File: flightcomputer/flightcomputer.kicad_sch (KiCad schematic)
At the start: 82 parts, among them J1 Conn_Coaxial, J10 Conn_01x03, J11 Conn_01x03, J12 ESQ-113-14-G-D, J13 Conn_01x07, J14 S3B-PH-K-S-GW, J15 B2P-VHLFSN, J2 Conn_Coaxial, J3 Conn_Coaxial, J4 Conn_Coaxial, J5 S3B-PH-K-S-GW, J6 Conn_01x03, J7 S4B-PH-K-S_LF__SN_, J8 Conn_01x03, J9 Conn_01x06, U1 MAX-M10S, U2 LIS2MDLTR, U3 BMI088, U4 MS5607-02BA, U5 ESP32-S3-WROOM-1-N4, U6 NCP718ASNADJT1G, U7 Teensy4.1, U8 LSM6DSO32TR, U9 RFM96W-433S2

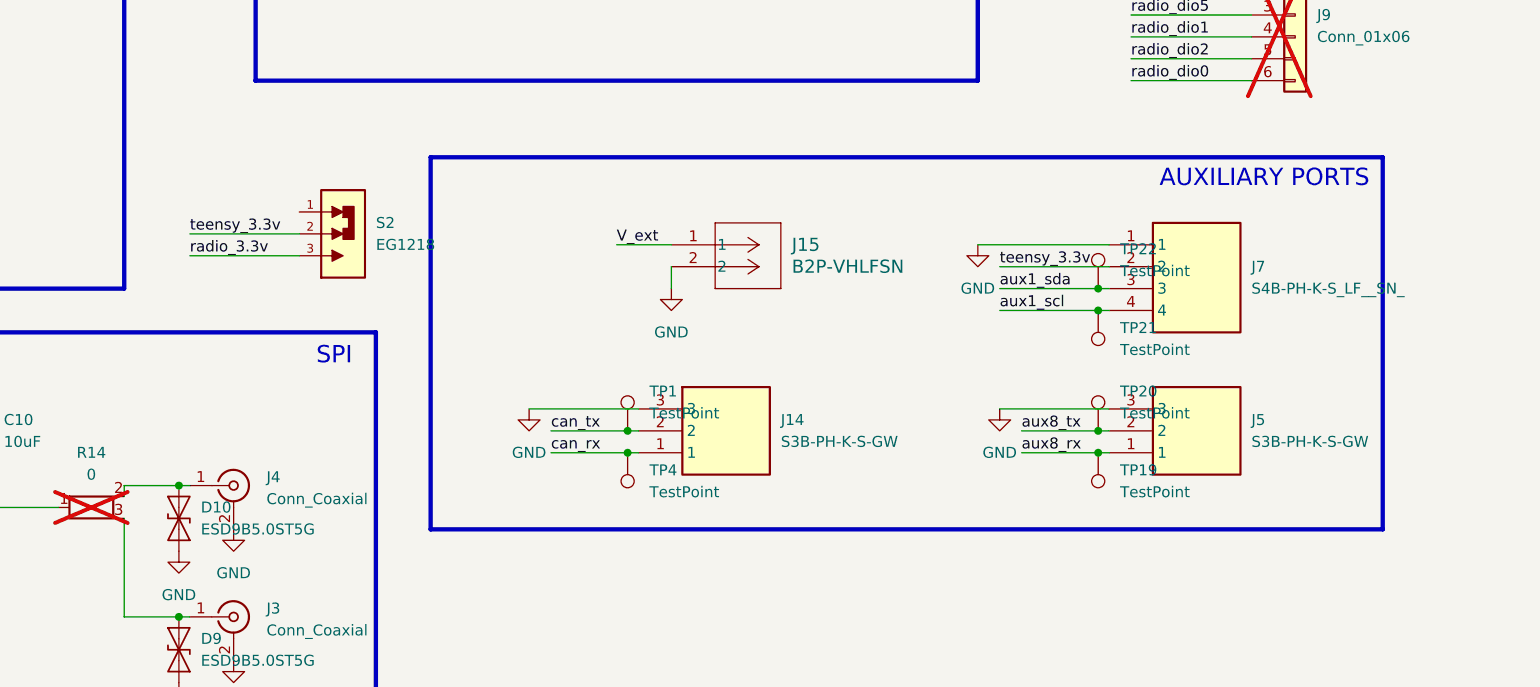
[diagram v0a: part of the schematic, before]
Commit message: prod files
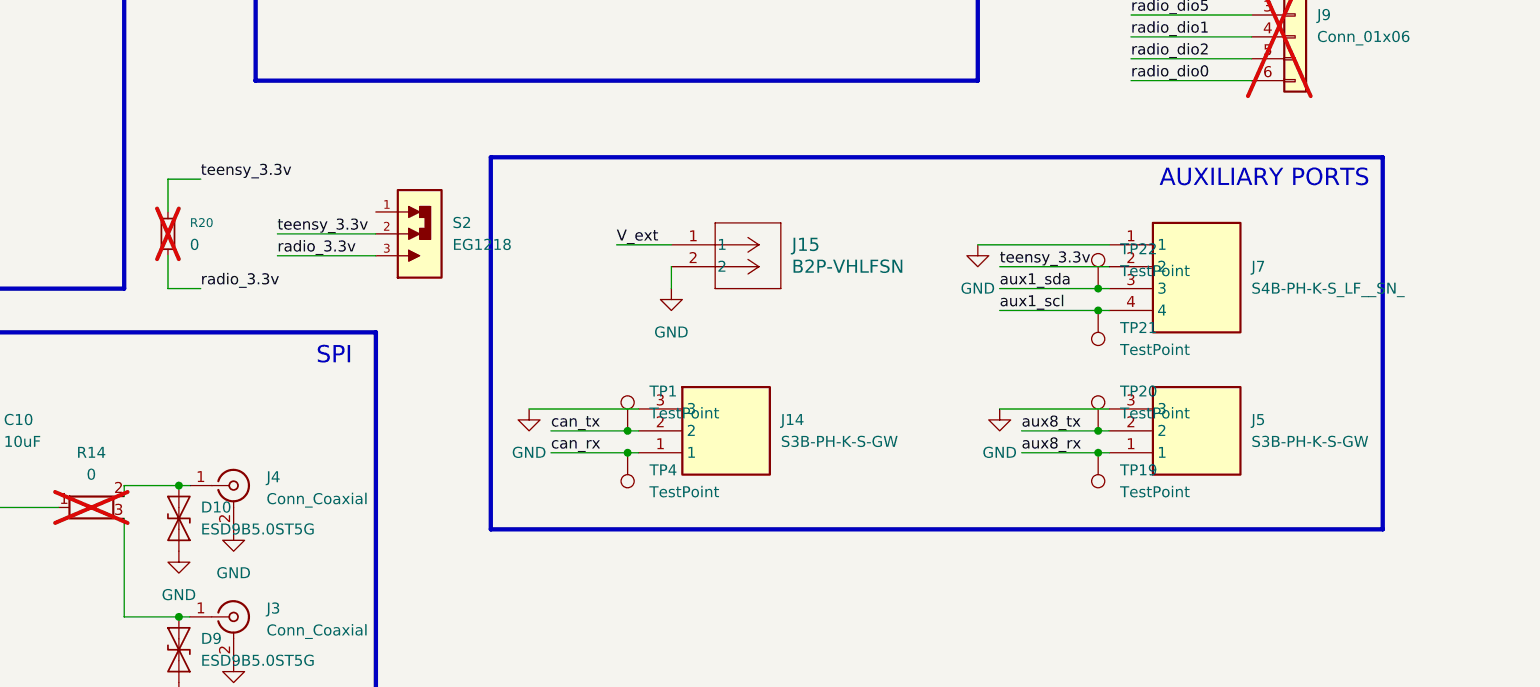
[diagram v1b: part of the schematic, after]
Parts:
- added R20: 0, Resistor_SMD:R_0603_1608Metric_Pad0.98x0.95mm_HandSolder, symbol Device:R_Small
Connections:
- net radio_3.3v: now also R20.2
- net teensy_3.3v: now also R20.1
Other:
- moved on the sheet: S2
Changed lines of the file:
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@@
 	)
 	(rectangle
-		(start 294.64 205.74)
+		(start 301.625 205.74)
 		(end 405.13 248.92)
 		(stroke
@@
 	(wire
 		(pts
-			(xy 266.7 217.17) (xy 279.4 217.17)
+			(xy 276.86 217.17) (xy 288.29 217.17)
 		)
 		(stroke
@@
 	(wire
 		(pts
+			(xy 264.16 220.98) (xy 267.97 220.98)
+		)
+		(stroke
+			(width 0)
+			(type default)
+		)
+	)
+	(wire
+		(pts
 			(xy 157.48 139.7) (xy 170.18 139.7)
 		)
@@
 	(wire
 		(pts
+			(xy 264.16 217.17) (xy 264.16 220.98)
+		)
+		(stroke
+			(width 0)
+			(type default)
+		)
+	)
+	(wire
+		(pts
 			(xy 226.06 152.4) (xy 240.03 152.4)
 		)
@@
 	(wire
 		(pts
+			(xy 264.16 208.28) (xy 267.97 208.28)
+		)
+		(stroke
+			(width 0)
+			(type default)
+		)
+	)
+	(wire
+		(pts
 			(xy 105.41 213.36) (xy 118.11 213.36)
 		)
@@
 	(wire
 		(pts
+			(xy 264.16 212.09) (xy 264.16 208.28)
+		)
+		(stroke
+			(width 0)
+			(type default)
+		)
+	)
+	(wire
+		(pts
 			(xy 226.06 124.46) (xy 240.03 124.46)
 		)
@@
 	(wire
 		(pts
-			(xy 266.7 214.63) (xy 279.4 214.63)
+			(xy 276.86 214.63) (xy 288.29 214.63)
 		)
 		(stroke
@@
 		)
 	)
+	(label "teensy_3.3v"
+		(at 267.97 208.28 0)
+		(effects
+			(font
+				(size 1.27 1.27)
+			)
+			(justify left bottom)
+		)
+	)
 	(label "GPS_int"
 		(at 240.03 127 180)
@@
 		)
 	)
+	(label "radio_3.3v"
+		(at 267.97 220.98 0)
+		(effects
+			(font
+				(size 1.27 1.27)
+			)
+			(justify left bottom)
+		)
+	)
 	(label "aux1_scl"
 		(at 231.14 139.7 0)
@@
 	)
 	(label "teensy_3.3v"
-		(at 266.7 214.63 0)
+		(at 276.86 214.63 0)
 		(effects
 			(font
@@
 	)
 	(label "radio_3.3v"
-		(at 266.7 217.17 0)
+		(at 276.86 217.17 0)
 		(effects
 			(font
@@
 	(symbol
 		(lib_id "HPRlibrary:EG1218")
-		(at 284.48 214.63 0)
+		(at 293.37 214.63 0)
 		(unit 1)
 		(exclude_from_sim no)
@@
 		(fields_autoplaced yes)
 		(property "Reference" "S2"
-			(at 288.29 213.3599 0)
+			(at 297.18 213.3599 0)
 			(effects
 				(font
@@
 		)
 		(property "Value" "EG1218"
-			(at 288.29 215.8999 0)
+			(at 297.18 215.8999 0)
 			(effects
 				(font
@@
 		)
 		(property "Footprint" "HPRlibrary:SW_EG1218"
-			(at 284.48 214.63 0)
+			(at 293.37 214.63 0)
 			(effects
 				(font
@@
 		)
 		(property "Datasheet" ""
-			(at 284.48 214.63 0)
+			(at 293.37 214.63 0)
 			(effects
 				(font
@@
 		)
 		(property "Description" "Slide Switch SPDT Through Hole"
-			(at 284.48 214.63 0)
+			(at 293.37 214.63 0)
 			(effects
 				(font
@@
 		)
 		(property "MF" "E-Switch"
-			(at 284.48 214.63 0)
+			(at 293.37 214.63 0)
 			(effects
 				(font
@@
 		)
 		(property "PACKAGE" "None"
-			(at 284.48 214.63 0)
+			(at 293.37 214.63 0)
 			(effects
 				(font
@@
 		)
 		(property "PRICE" "None"
-			(at 284.48 214.63 0)
+			(at 293.37 214.63 0)
 			(effects
 				(font
@@
 		)
 		(property "MP" "EG1218"
-			(at 284.48 214.63 0)
+			(at 293.37 214.63 0)
 			(effects
 				(font
@@
 		)
 		(property "AVAILABILITY" "In Stock"
-			(at 284.48 214.63 0)
+			(at 293.37 214.63 0)
 			(effects
 				(font
@@
 		)
 		(property "PURCHASE-URL" "https://pricing.snapeda.com/search/part/EG1218/?ref=eda"
-			(at 284.48 214.63 0)
+			(at 293.37 214.63 0)
 			(effects
 				(font
@@
 					(unit 1)
 				)
+			)
+		)
+	)
+	(symbol
+		(lib_id "Device:R_Small")
+		(at 264.16 214.63 0)
+		(unit 1)
+		(exclude_from_sim no)
+		(in_bom yes)
+		(on_board yes)
+		(dnp yes)
+		(fields_autoplaced yes)
+		(property "Reference" "R20"
+			(at 266.7 213.3599 0)
+			(effects
+				(font
+					(size 1.016 1.016)
+				)
+				(justify left)
+			)
+		)
+		(property "Value" "0"
+			(at 266.7 215.8999 0)
+			(effects
+				(font
+					(size 1.27 1.27)
+				)
+				(justify left)
+			)
+		)
+		(property "Footprint" "Resistor_SMD:R_0603_1608Metric_Pad0.98x0.95mm_HandSolder"
+			(at 264.16 214.63 0)
+			(effects
+				(font
+					(size 1.27 1.27)
+				)
+				(hide yes)
+			)
+		)
+		(property "Datasheet" "~"
+			(at 264.16 214.63 0)
+			(effects
+				(font
+					(size 1.27 1.27)
+				)
+				(hide yes)
+			)
+		)
+		(property "Description" "Resistor, small symbol"
+			(at 264.16 214.63 0)
+			(effects
+				(font
+					(size 1.27 1.27)
+				)
+				(hide yes)
+			)
+		)
+		(pin "1"
+		)
+		(pin "2"
+		)
+		(instances
+			(project ""
+				(path "/7ffad011-bb39-4f19-b4f2-0143f1626449"
+					(reference "R20")
+					(unit 1)
+				)
